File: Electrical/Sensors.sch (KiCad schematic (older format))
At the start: 2 parts

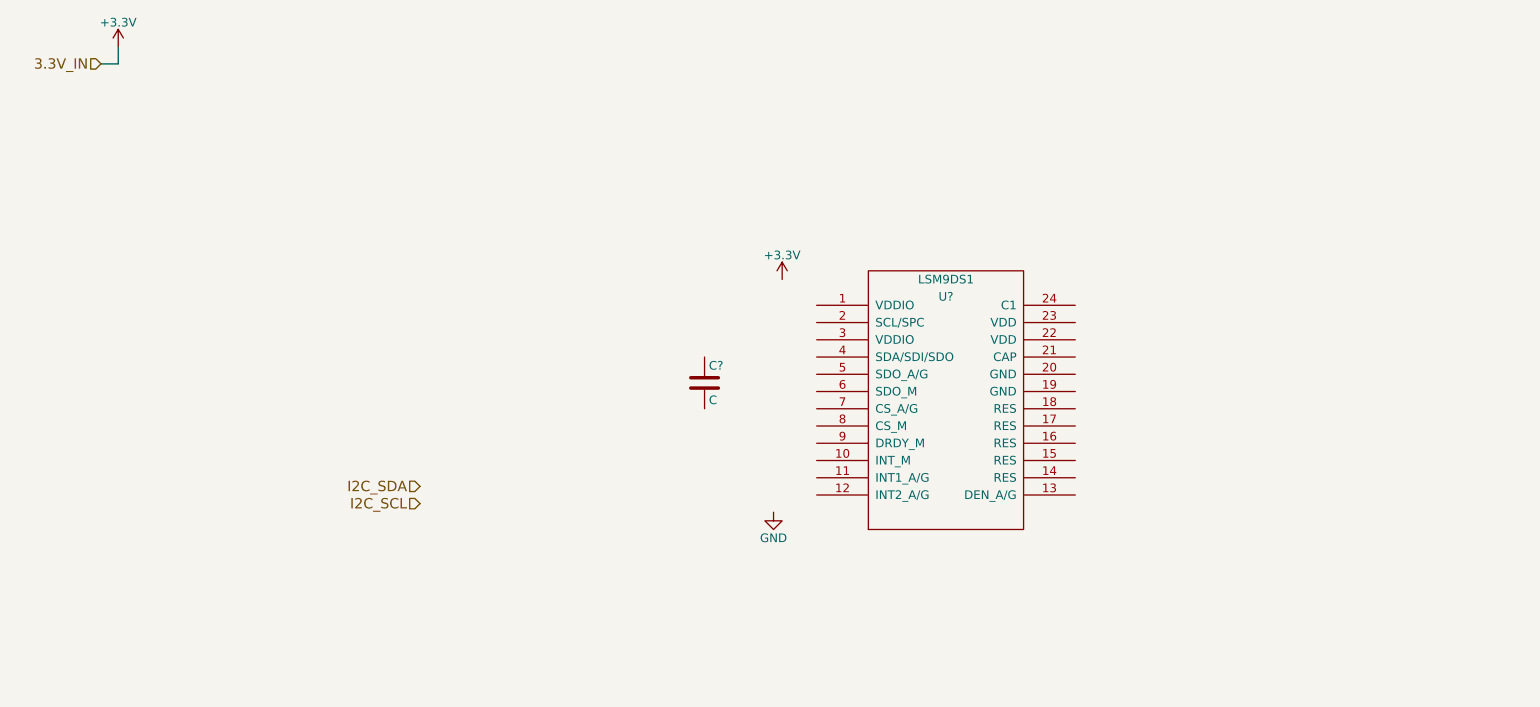
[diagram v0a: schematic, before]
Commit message: Finished sensor sheet
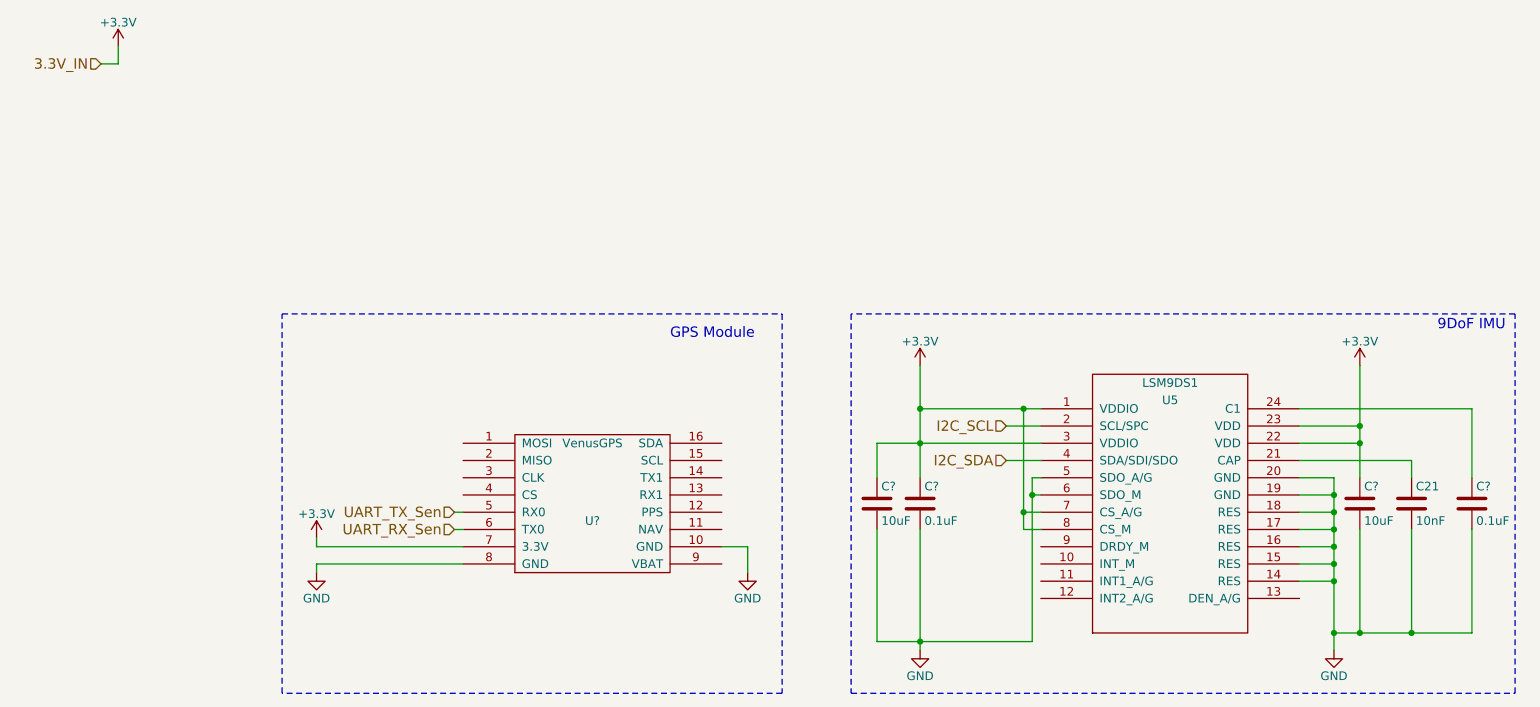
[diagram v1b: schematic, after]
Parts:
- added C? (x2): 0.1uF, symbol C
- added C? (x2): 10uF, symbol C
- added U?: VenusGPS, MODULE, symbol VenusGPS
- C21: renamed from C?; value C -> 10nF
- gave numbers to parts that had none: 1
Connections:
- net +3V3: now also U5.1 (VDDIO), U5.22 (VDD), U5.23 (VDD), U5.3 (VDDIO), U5.7 (CS_A/G), U5.8 (CS_M), C?.1, C?.1, C?.1, U?.7 (3.3V)
- net GND: now also C21.2, U5.14 (RES), U5.15 (RES), U5.16 (RES), U5.17 (RES), U5.18 (RES), U5.19 (GND), U5.20 (GND), U5.5 (SDO_A/G), U5.6 (SDO_M), C?.2, C?.2, C?.2, C?.2, U?.10 (GND), U?.8 (GND)
- net I2C_SCL: now also U5.2 (SCL/SPC)
- net I2C_SDA: now also U5.4 (SDA/SDI/SDO)
- net at U5.21 (CAP): now also C21.1
- net at U5.24 (C1): now also C?.1
- new net UART_RX_Sen: U?.6 (TX0)
- new net UART_TX_Sen: U?.5 (RX0)
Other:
- note added: "9DoF IMU"
- note added: "GPS Module"
- moved on the sheet: C21, U5
